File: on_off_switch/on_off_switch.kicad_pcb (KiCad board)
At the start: 2 copper layers, 17 parts, among them K1 HFD23_005-1ZS, Q1 BC846, U1 ATtiny13A-P, U2 L78L05_SOT89

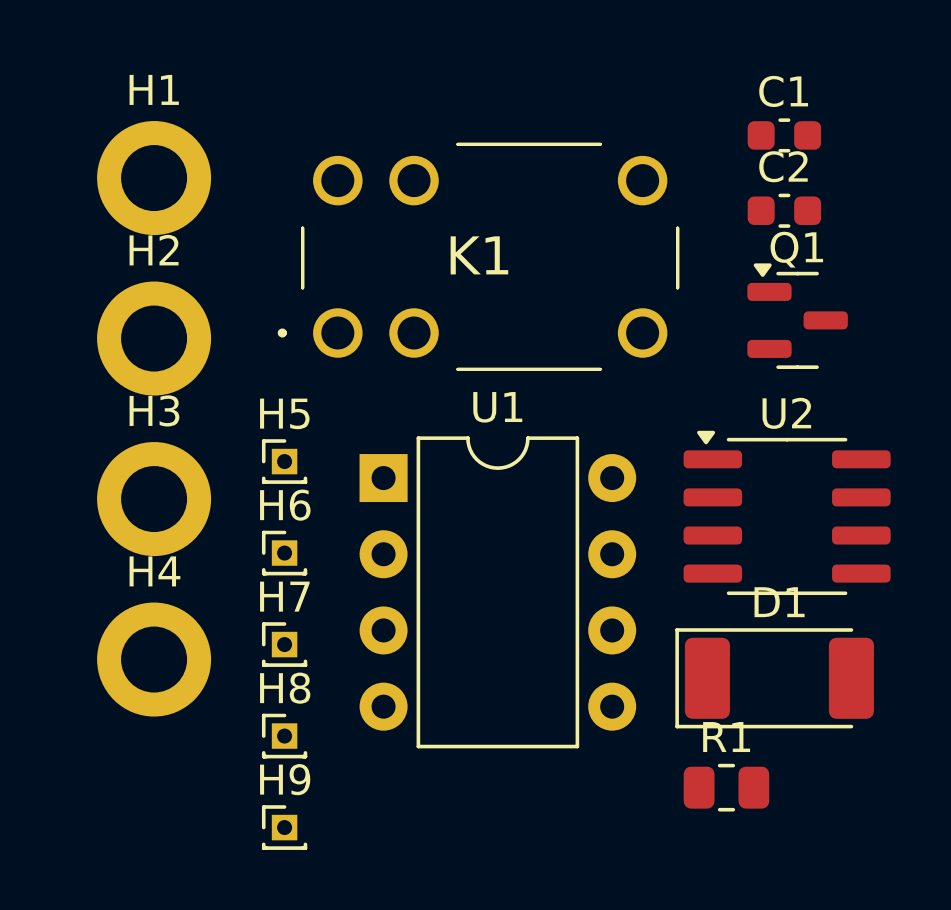
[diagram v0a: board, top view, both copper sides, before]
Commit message: added PCB design
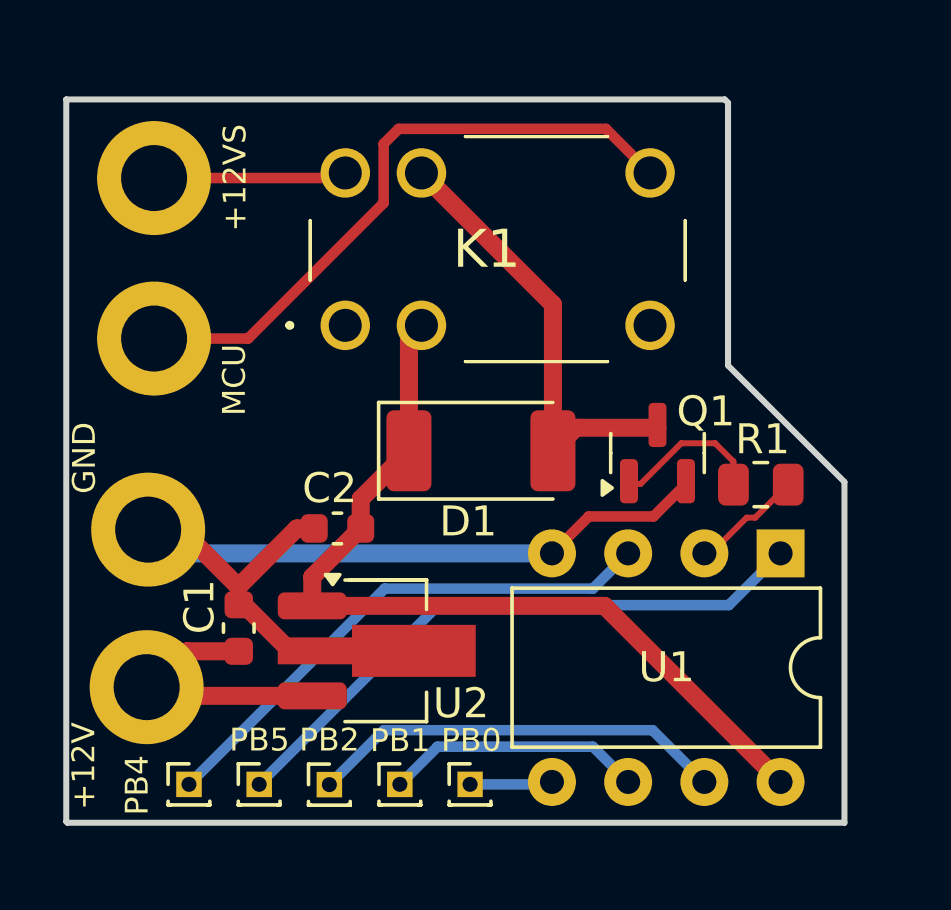
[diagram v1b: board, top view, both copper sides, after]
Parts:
- U2: footprint Package_SO:SOIC-8_3.9x4.9mm_P1.27mm -> Package_TO_SOT_SMD:SOT-89-3_Handsoldering
- moved C1 24.5 mm to (121.6, 65.6), turned to 90 degrees
- moved C2 18.3 mm to (124.9, 62.3), turned to 180 degrees
- moved U2 14.1 mm to (126.5, 66.4)
- moved U1 13.5 mm to (139.7, 63.1), turned to -90 degrees
- moved D1 12.5 mm to (129.7, 59.7)
- moved PB0 12.4 mm to (129.3, 70.8)
- moved R1 10.2 mm to (139.0, 60.9), turned to 180 degrees
- moved PB1 8.61 mm to (127.0, 70.8)
- moved Q1 6.43 mm to (135.6, 59.8), turned to 90 degrees
- moved PB2 4.90 mm to (124.6, 70.8)
- moved PB4 3.57 mm to (119.9, 70.8)
- moved PB5 1.67 mm to (122.3, 70.8)
- moved GND 1.04 mm to (118.6, 62.4)
- moved +12V 0.95 mm to (118.5, 67.6)
- moved K1 0.36 mm to (125.2, 55.5)
- renumbered H4 to +12V, H1 to +12VS, H3 to GND, H2 to MCU, H5 to PB0, H6 to PB1, H7 to PB2, H8 to PB4, H9 to PB5
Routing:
- net GND: track 0.00 -> 30.3 mm
- net +5V: track 0.00 -> 28.9 mm
- net MCU_PIN_AS&G: track 0.00 -> 21.2 mm
- net Net-(U1-~{RESET}/PB5): track 0.00 -> 20.6 mm
- net Net-(U1-PB4): track 0.00 -> 17.8 mm
- net Net-(D1-A): track 0.00 -> 14.9 mm
- net Net-(U1-PB2): track 0.00 -> 14.0 mm
- net +12V: track 0.00 -> 10.6 mm
- net Net-(U1-PB1): track 0.00 -> 8.62 mm
- net 12VSIGNAL_PIN_AS&G: track 0.00 -> 6.44 mm
- net Net-(Q1-B): track 0.00 -> 5.07 mm
- net base_signal: track 0.00 -> 3.74 mm
- net Net-(U1-PB0): track 0.00 -> 2.76 mm
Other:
- board outline added: 25.9 x 24.1 mm
